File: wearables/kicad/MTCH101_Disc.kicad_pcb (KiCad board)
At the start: 2 copper layers, 25.4 x 25.4 mm, 15 parts, among them U1 MTCH101

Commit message: reworking.
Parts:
- U1: value MTCH101 -> MTCH101_PKG
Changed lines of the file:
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@@
       (effects (font (size 1 1) (thickness 0.15)))
     )
-    (fp_text value MTCH101 (at 0 2.9) (layer F.Fab)
+    (fp_text value MTCH101_PKG (at 0 2.9) (layer F.Fab)
       (effects (font (size 1 1) (thickness 0.15)))
     )

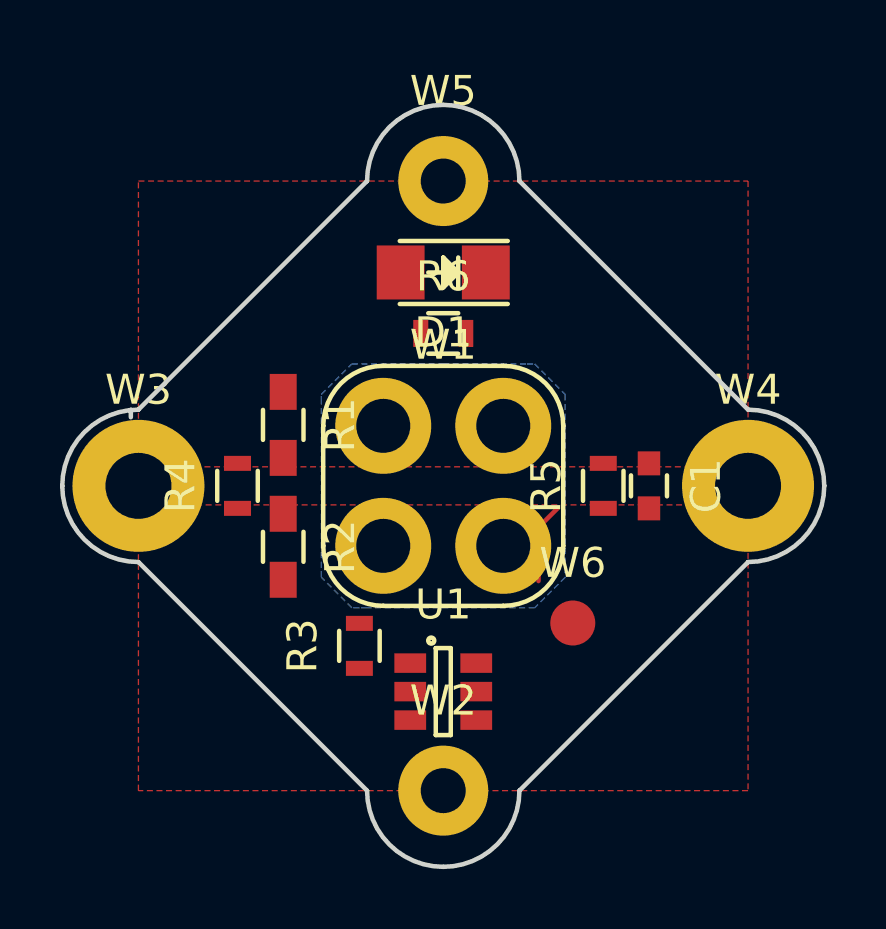
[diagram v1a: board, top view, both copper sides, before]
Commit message: exploring vdd/gnd routing options
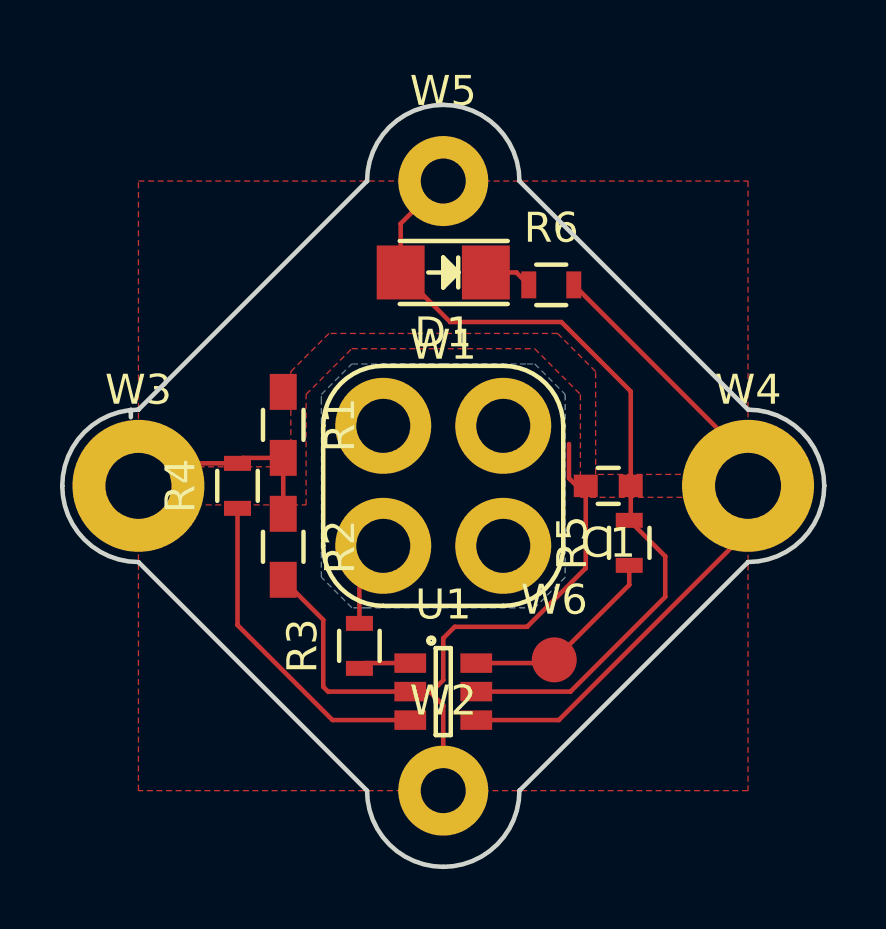
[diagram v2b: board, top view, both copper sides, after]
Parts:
- moved R6 3.95 mm to (128.1, 89.1)
- moved R5 2.09 mm to (130.7, 97.7)
- moved W6 1.37 mm to (128.2, 101.6)
- moved C1 1.36 mm to (130.0, 95.8), turned to 180 degrees
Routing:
- net VDD: track 0.00 -> 27.9 mm
- net GND: track 0.00 -> 24.1 mm
- net /out: track 0.00 -> 21.8 mm
- net /MTSA: track 0.00 -> 11.0 mm
- net /ref: track 0.00 -> 7.08 mm
- net /pm: track 0.00 -> 6.68 mm
- net /MTI: track 0.00 -> 1.77 mm
- net Net-(D1-Pad1): track 0.00 -> 1.60 mm
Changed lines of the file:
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@@
   (general
     (links 22)
-    (no_connects 18)
-    (area 111.684999 82.982999 137.235001 108.533001)
+    (no_connects 0)
+    (area 93.444287 71.468 138.32002 109.9454)
     (thickness 1.6002)
     (drawings 17)
-    (tracks 2)
+    (tracks 49)
     (zones 0)
     (modules 15)
@@
   )
   (module Capacitors_SMD:C_0603 (layer Top)
-    (at 131.318 95.758 270)
+    (at 129.96 95.758 180)
     (descr "Capacitor SMD 0603, reflow soldering, AVX (see smccp.pdf)")
     (tags "capacitor 0603")
     (attr smd)
-    (fp_text reference C1 (at 0 -1.9 270) (layer F.SilkS)
-      (effects (font (size 1 1) (thickness 0.15)))
-    )
-    (fp_text value 0.1u (at 0 1.9 270) (layer F.Fab)
+    (fp_text reference C1 (at 0 -1.9 180) (layer F.SilkS)
+      (effects (font (size 1 1) (thickness 0.15)))
+    )
+    (fp_text value 0.1u (at 0 1.9 180) (layer F.Fab)
       (effects (font (size 1 1) (thickness 0.15)))
     )
@@
     (fp_line (start -0.35 -0.6) (end 0.35 -0.6) (layer F.SilkS) (width 0.15))
     (fp_line (start 0.35 0.6) (end -0.35 0.6) (layer F.SilkS) (width 0.15))
-    (pad 1 smd rect (at -0.75 0 270) (size 0.8 0.75) (layers Top F.Paste F.Mask)
+    (pad 1 smd rect (at -0.75 0 180) (size 0.8 0.75) (layers Top F.Paste F.Mask)
       (net 1 VDD))
-    (pad 2 smd rect (at 0.75 0 270) (size 0.8 0.75) (layers Top F.Paste F.Mask)
+    (pad 2 smd rect (at 0.75 0 180) (size 0.8 0.75) (layers Top F.Paste F.Mask)
       (net 2 GND))
     (model Capacitors_SMD.3dshapes/C_0603.wrl
@@
   )
   (module Resistors_SMD:R_0603 (layer Top)
-    (at 129.794 95.758 90)
+    (at 130.66 97.658 90)
     (descr "Resistor SMD 0603, reflow soldering, Vishay (see dcrcw.pdf)")
     (tags "resistor 0603")
@@
   )
   (module Resistors_SMD:R_0603 (layer Top)
-    (at 124.46 90.678)
+    (at 128.06 89.058)
     (descr "Resistor SMD 0603, reflow soldering, Vishay (see dcrcw.pdf)")
     (tags "resistor 0603")
@@
   )
   (module Measurement_Points:Measurement_Point_Round-SMD-Pad_Small (layer Top)
-    (at 128.778 100.33)
+    (at 128.16 101.558)
     (descr "Mesurement Point, Round, SMD Pad, DM 1.5mm,")
     (tags "Mesurement Point Round SMD Pad 1.5mm")
@@
     (arrow2b (pts (xy 100.33 108.458) (xy 99.743579 107.331496)))
   )
-  (segment (start 127.635 98.933) (end 127.635 97.143) (width 0.1524) (layer Top) (net 6))
-  (segment (start 127.635 97.143) (end 128.27 96.508) (width 0.1524) (layer Top) (net 6))
-  (zone (net 1) (net_name VDD) (layer Top) (hatch edge 0.508)
-    (connect_pads (clearance 0.508))
-    (min_thickness 0.254)
-    (fill yes (arc_segments 16) (thermal_gap 0.508) (thermal_bridge_width 0.508))
-    (polygon
-      (pts
-        (xy 134.62 95.123) (xy 114.3 95.123) (xy 114.3 85.598) (xy 134.62 85.598)
-      )
-    )
-  )
+  (segment (start 130.71 95.758) (end 130.71 92.61) (width 0.1524) (layer Top) (net 1))
+  (segment (start 124.69114 90.297) (end 123.04014 88.646) (width 0.1524) (layer Top) (net 1))
+  (segment (start 128.397 90.297) (end 124.69114 90.297) (width 0.1524) (layer Top) (net 1))
+  (segment (start 130.71 92.61) (end 128.397 90.297) (width 0.1524) (layer Top) (net 1))
+  (segment (start 131.86 99.458) (end 131.86 98.108) (width 0.1524) (layer Top) (net 1))
+  (segment (start 128.702 102.616) (end 131.86 99.458) (width 0.1524) (layer Top) (net 1))
+  (segment (start 125.56 102.616) (end 128.702 102.616) (width 0.1524) (layer Top) (net 1))
+  (segment (start 131.86 98.108) (end 130.71 96.958) (width 0.1524) (layer Top) (net 1))
+  (segment (start 130.71 96.958) (end 130.71 95.758) (width 0.1524) (layer Top) (net 1))
+  (segment (start 123.04014 88.646) (end 123.04014 87.01786) (width 0.1524) (layer Top) (net 1))
+  (segment (start 123.04014 87.01786) (end 124.46 85.598) (width 0.1524) (layer Top) (net 1))
+  (segment (start 129.21 95.758) (end 128.905 95.758) (width 0.1524) (layer Top) (net 2))
+  (segment (start 128.905 95.758) (end 128.651 95.504) (width 0.1524) (layer Top) (net 2))
+  (segment (start 128.651 95.504) (end 128.651 94.361) (width 0.1524) (layer Top) (net 2))
+  (segment (start 123.36 102.616) (end 124.079 102.616) (width 0.1524) (layer Top) (net 2))
+  (segment (start 129.21 98.501) (end 129.21 95.758) (width 0.1524) (layer Top) (net 2))
+  (segment (start 127.254 100.457) (end 129.21 98.501) (width 0.1524) (layer Top) (net 2))
+  (segment (start 124.841 100.457) (end 127.254 100.457) (width 0.1524) (layer Top) (net 2))
+  (segment (start 124.46 100.838) (end 124.841 100.457) (width 0.1524) (layer Top) (net 2))
+  (segment (start 124.46 102.235) (end 124.46 100.838) (width 0.1524) (layer Top) (net 2))
+  (segment (start 124.079 102.616) (end 124.46 102.235) (width 0.1524) (layer Top) (net 2))
+  (segment (start 124.46 105.918) (end 124.46 103.074) (width 0.1524) (layer Top) (net 2))
+  (segment (start 124.46 103.074) (end 124.002 102.616) (width 0.1524) (layer Top) (net 2))
+  (segment (start 123.36 102.616) (end 124.002 102.616) (width 0.1524) (layer Top) (net 2))
+  (segment (start 123.36 102.616) (end 120.618 102.616) (width 0.1524) (layer Top) (net 2))
+  (segment (start 120.46 100.224) (end 119.126 98.89) (width 0.1524) (layer Top) (net 2))
+  (segment (start 120.46 102.458) (end 120.46 100.224) (width 0.1524) (layer Top) (net 2))
+  (segment (start 120.618 102.616) (end 120.46 102.458) (width 0.1524) (layer Top) (net 2))
+  (segment (start 125.87986 88.646) (end 126.898 88.646) (width 0.1524) (layer Top) (net 3))
+  (segment (start 126.898 88.646) (end 127.31 89.058) (width 0.1524) (layer Top) (net 3))
+  (segment (start 117.602 95.008) (end 115.05 95.008) (width 0.1524) (layer Top) (net 4))
+  (segment (start 115.05 95.008) (end 114.3 95.758) (width 0.1524) (layer Top) (net 4))
+  (segment (start 119.126 94.826) (end 117.784 94.826) (width 0.1524) (layer Top) (net 4))
+  (segment (start 117.784 94.826) (end 117.602 95.008) (width 0.1524) (layer Top) (net 4))
+  (segment (start 119.126 94.826) (end 119.126 96.69) (width 0.1524) (layer Top) (net 4))
+  (segment (start 123.36 101.666) (end 121.842 101.666) (width 0.1524) (layer Top) (net 5))
+  (segment (start 121.842 101.666) (end 121.666 101.842) (width 0.1524) (layer Top) (net 5))
+  (segment (start 121.666 100.342) (end 121.666 98.552) (width 0.1524) (layer Top) (net 6))
+  (segment (start 121.666 98.552) (end 122.46 97.758) (width 0.1524) (layer Top) (net 6))
+  (segment (start 123.36 103.566) (end 120.768 103.566) (width 0.1524) (layer Top) (net 7))
+  (segment (start 117.602 100.4) (end 117.602 96.508) (width 0.1524) (layer Top) (net 7))
+  (segment (start 120.768 103.566) (end 117.602 100.4) (width 0.1524) (layer Top) (net 7))
+  (segment (start 130.66 98.408) (end 130.66 99.058) (width 0.1524) (layer Top) (net 8))
+  (segment (start 130.66 99.058) (end 128.16 101.558) (width 0.1524) (layer Top) (net 8))
+  (segment (start 125.56 101.666) (end 128.052 101.666) (width 0.1524) (layer Top) (net 8))
+  (segment (start 134.62 95.758) (end 134.62 94.868) (width 0.1524) (layer Top) (net 9))
+  (segment (start 134.62 94.868) (end 128.81 89.058) (width 0.1524) (layer Top) (net 9))
+  (segment (start 125.56 103.566) (end 128.312 103.566) (width 0.1524) (layer Top) (net 9))
+  (segment (start 128.312 103.566) (end 135.37 96.508) (width 0.1524) (layer Top) (net 9))
   (zone (net 2) (net_name GND) (layer Top) (hatch edge 0.508)
     (connect_pads (clearance 0.508))
@@
     (polygon
       (pts
-        (xy 134.62 105.918) (xy 114.3 105.918) (xy 114.3 96.393) (xy 134.62 96.393)
+        (xy 129.032 92.71) (xy 129.032 96.139) (xy 134.62 96.139) (xy 134.62 105.918) (xy 114.3 105.918)
+        (xy 114.3 96.393) (xy 119.888 96.393) (xy 119.888 92.71) (xy 121.412 91.186) (xy 127.508 91.186)
       )
     )
@@
       )
     )
+  )
+  (zone (net 1) (net_name VDD) (layer Top) (hatch edge 0.508)
+    (connect_pads (clearance 0.508))
+    (min_thickness 0.254)
+    (fill yes (arc_segments 16) (thermal_gap 0.508) (thermal_bridge_width 0.508))
+    (polygon
+      (pts
+        (xy 134.62 95.377) (xy 129.54 95.377) (xy 129.54 91.948) (xy 128.27 90.678) (xy 120.65 90.678)
+        (xy 119.38 91.948) (xy 119.38 95.123) (xy 114.3 95.123) (xy 114.3 85.598) (xy 134.62 85.598)
+      )
+    )
